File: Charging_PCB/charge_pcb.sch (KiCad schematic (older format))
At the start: 35 parts, among them J1 PCB_1, J2 Battery, J3 Power Switch, J4 24V Out, J5 Motor_Left, J6 Motor_Cutter, J7 Motor_Right, Q1 BC547C, Q2 IRLB 8721, Q3 BC547C, Q4 IRLB 8721, U1 ACS712

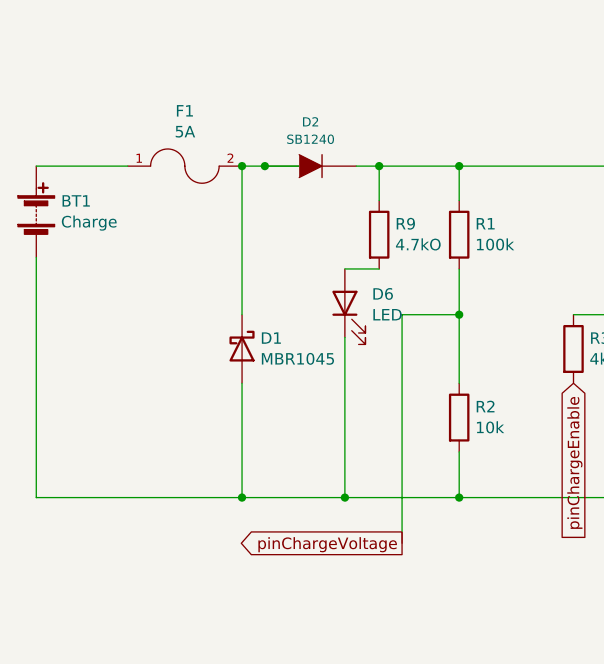
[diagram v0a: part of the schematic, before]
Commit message: PCB Changes
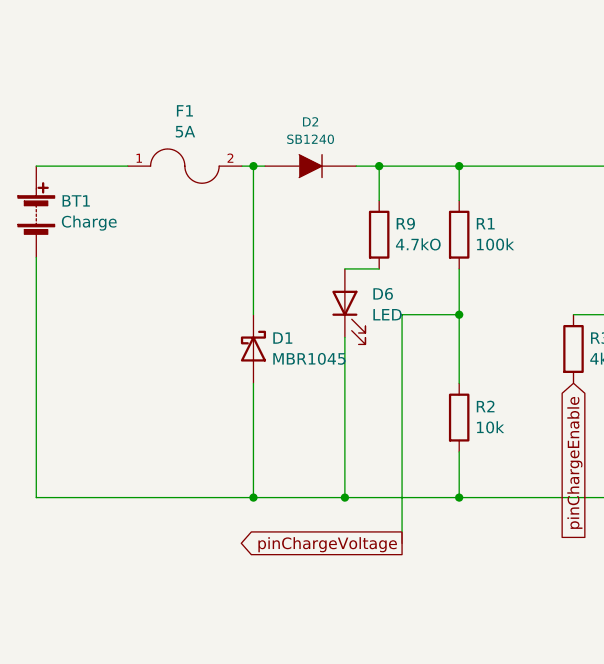
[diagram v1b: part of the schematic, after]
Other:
- moved on the sheet: D1
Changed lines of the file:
@@
 	2500 2250 2500 2400
 Wire Wire Line
-	1550 2250 1650 2250
+	1550 2250 1600 2250
 Wire Wire Line
 	2500 2700 2500 2900
@@
 	6500 3050 6550 3050
 Connection ~ 6500 2400
-Connection ~ 1550 2250
-Connection ~ 1550 3700
-Wire Wire Line
-	1550 3700 650  3700
-Wire Wire Line
-	1550 3700 2000 3700
 Text GLabel 2250 3900 0    50   Output ~ 0
 pinChargeVoltage
 Wire Wire Line
-	1550 3200 1550 3700
-Wire Wire Line
-	1550 2250 1550 2900
+	1600 3200 1600 3700
+Wire Wire Line
+	1600 2250 1600 2900
 $Comp
 L Diode:MBR745 D1
 U 1 1 60702097
-P 1550 3050
-F 0 "D1" V 1504 3130 50  0000 L CNN
-F 1 "MBR1045" V 1595 3130 50  0000 L CNN
-F 2 "Package_TO_SOT_THT:TO-220-2_Vertical" H 1550 2875 50  0001 C CNN
-F 3 "http://www.onsemi.com/pub_link/Collateral/MBR735-D.PDF" H 1550 3050 50  0001 C CNN
-	1    1550 3050
+P 1600 3050
+F 0 "D1" V 1554 3130 50  0000 L CNN
+F 1 "MBR1045" V 1645 3130 50  0000 L CNN
+F 2 "Package_TO_SOT_THT:TO-220-2_Vertical" H 1600 2875 50  0001 C CNN
+F 3 "http://www.onsemi.com/pub_link/Collateral/MBR735-D.PDF" H 1600 3050 50  0001 C CNN
+	1    1600 3050
 	0    1    1    0
 $EndComp
@@
 Wire Wire Line
 	2250 2900 2500 2900
-Connection ~ 1650 2250
-Wire Wire Line
-	1650 2250 1800 2250
 Wire Wire Line
 	2050 2250 2150 2250
@@
 	1    0    0    -1
 $EndComp
+Connection ~ 1600 2250
+Connection ~ 1600 3700
+Wire Wire Line
+	1600 3700 2000 3700
+Wire Wire Line
+	650  3700 1600 3700
+Wire Wire Line
+	1600 2250 1650 2250
 $EndSCHEMATC
